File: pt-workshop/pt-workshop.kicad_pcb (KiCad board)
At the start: 2 copper layers, 22.9 x 48.3 mm, 39 parts, among them J101 Conn_01x10, J102 Conn_01x10, Q301 NST65011, U201 L78L05, U202 PT2399-Detailed, U301 TL972

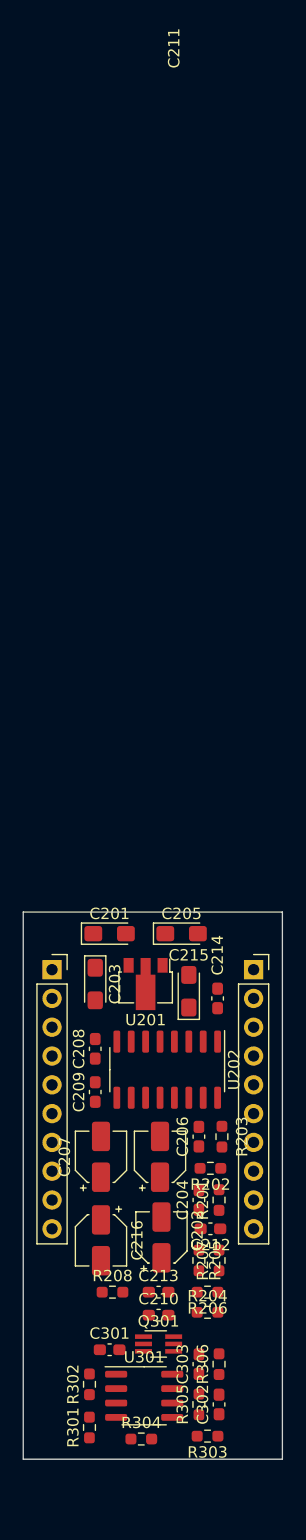
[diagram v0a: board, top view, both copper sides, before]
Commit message: Board layed out
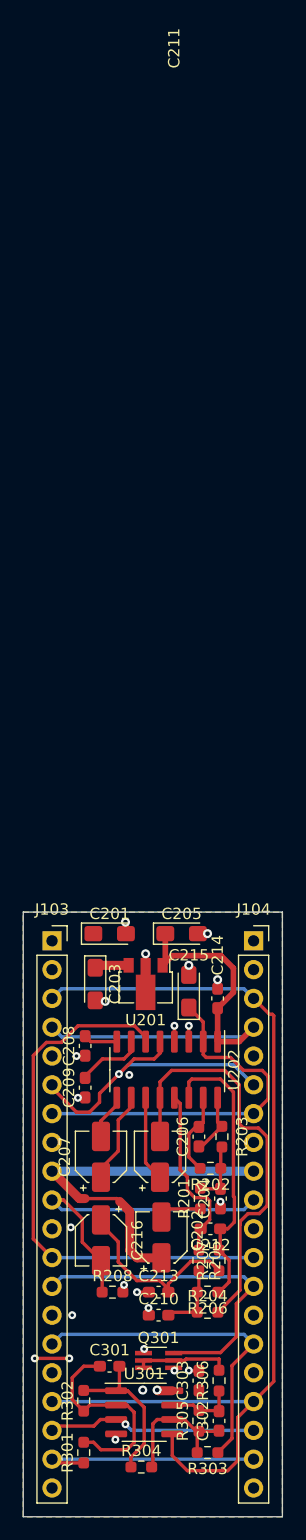
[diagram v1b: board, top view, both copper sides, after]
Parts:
- removed J101, J102: Conn_01x10, Connector_PinSocket_2.54mm:PinSocket_1x10_P2.54mm_Vertical
- added J103: Conn_01x20, Connector_PinSocket_2.54mm:PinSocket_1x20_P2.54mm_Vertical, F.Cu at (27.9, 58.4)
- added J104: Conn_01x20, Connector_PinSocket_2.54mm:PinSocket_1x20_P2.54mm_Vertical, F.Cu at (45.7, 58.4)
- moved R304 2.47 mm to (35.8, 104.8)
- moved R301 2.27 mm to (30.7, 103.6)
- moved C204 1.91 mm to (42.8, 81.2)
- moved R201 1.66 mm to (41.0, 81.2)
- moved R302 1.54 mm to (30.7, 99.0)
- moved C302 1.45 mm to (42.7, 100.8)
- moved C303 1.45 mm to (40.9, 97.2)
- moved R305 1.45 mm to (40.9, 100.8)
- moved R306 1.45 mm to (42.7, 97.2)
- moved C301 1.45 mm to (33.0, 95.9)
- moved Q301 1.45 mm to (37.3, 95.4)
- moved R303 1.45 mm to (41.7, 103.6)
- moved U301 1.45 mm to (36.1, 100.0)
- moved C209 0.97 mm to (30.9, 71.4)
- moved C208 0.92 mm to (30.9, 67.7)
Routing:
- net /PT_4.5V: track 0.00 -> 87.8 mm
- net /PT_Ic: track 0.00 -> 48.1 mm
- net /PT_5V: track 0.00 -> 39.2 mm
- net /PT2399-adapter/DEMOD_OUT: track 0.00 -> 37.0 mm
- net /PT_Ref: track 0.00 -> 32.8 mm
- net /PT_In: track 0.00 -> 32.6 mm
- net /PT_Iout: track 0.00 -> 29.7 mm
- net /PT_Voffset: track 0.00 -> 29.4 mm
- net /PT_Out: track 0.00 -> 29.0 mm
- net /PT_CLK: track 0.00 -> 27.2 mm, vias 0 -> 1
- net Net-(C212-Pad1): track 0.00 -> 25.4 mm
- net /PT_AttVert3: track 0.00 -> 20.7 mm
- net Net-(C301-Pad1): track 0.00 -> 18.8 mm
- net /PT_AttVert2: track 0.00 -> 17.6 mm, vias 0 -> 1
- net Net-(C213-Pad2): track 0.00 -> 16.4 mm
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- added copper zone on B.Cu, net /PT_9V
- added copper zone on F.Cu, net /PT_9V
- added copper zone on In1.Cu, net /PT_GND
- added copper zone on In2.Cu, net /PT_GND
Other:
- board size 22.9 x 48.3 mm -> 22.9 x 53.3 mm
- copper layers 2 -> 4

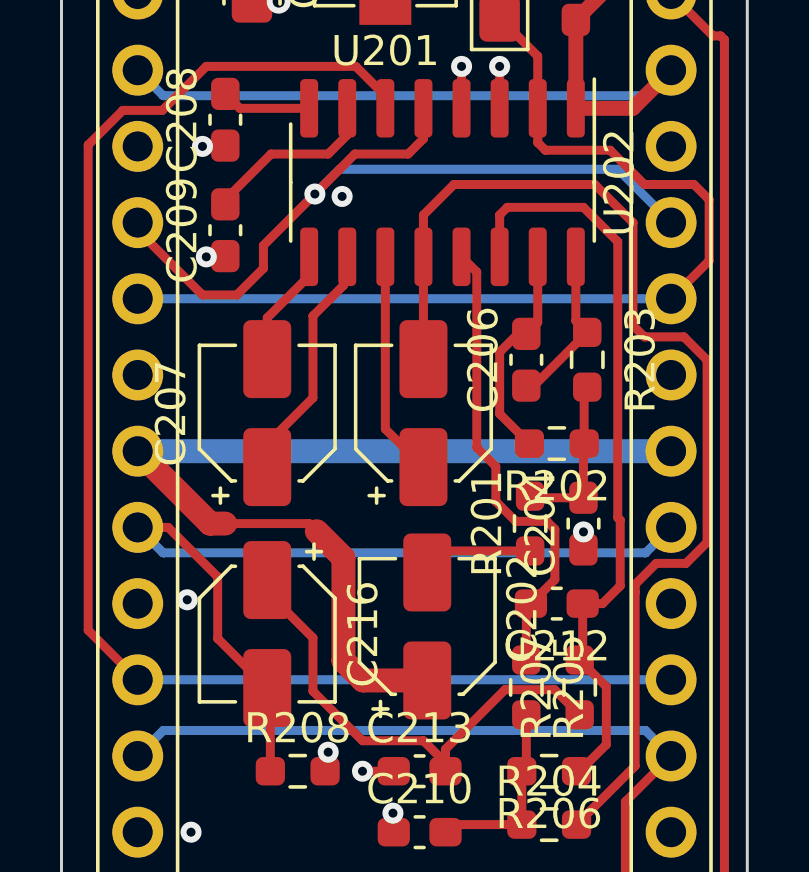
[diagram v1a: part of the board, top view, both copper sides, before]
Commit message: wip
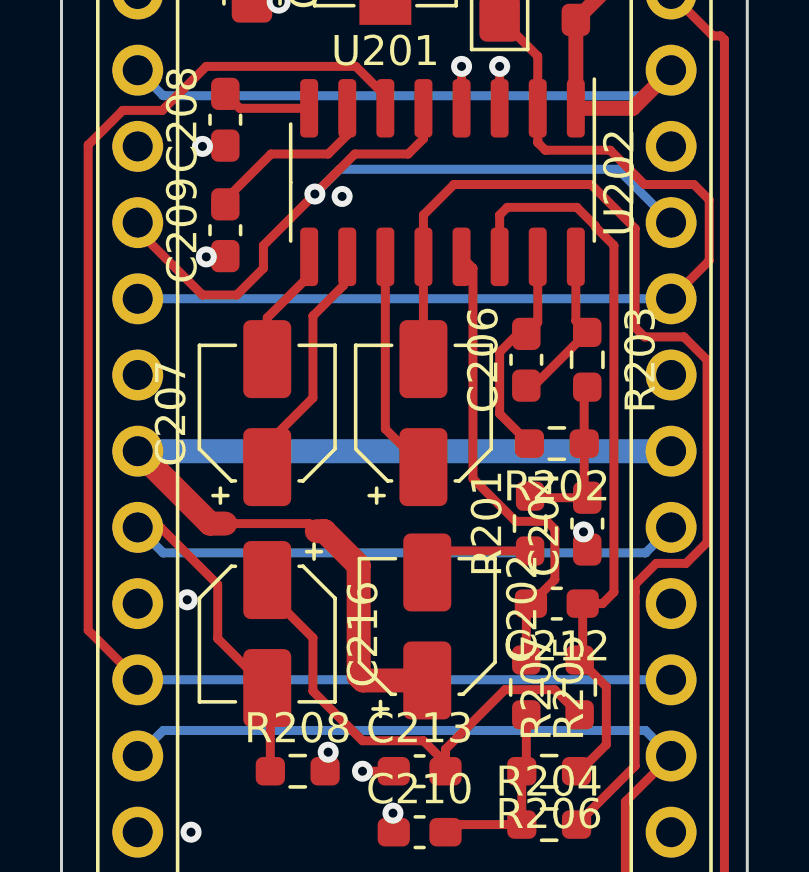
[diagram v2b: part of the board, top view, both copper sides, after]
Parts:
- moved C204 0.13 mm to (42.9, 81.2)
